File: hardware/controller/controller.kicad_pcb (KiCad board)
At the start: 2 copper layers, 150 x 68 mm, 142 parts, among them J1 Conn_01x05, J2 Conn_01x03, J3 Conn_01x04, J4 USB_B_Micro, J5 Conn_01x03, SW1 ILS_TA180_50, SW10 SW_SPDT, SW2 ILS_TA180_50, SW3 ILS_TA180_50, SW4 ILS_TA180_50, SW5 ILS_TA180_50, SW6 ILS_TA180_50, SW7 ILS_TA180_50, SW8 ILS_TA180_50, SW9 ILS_TA180_50, U1 WS2811, U2 STM32F103C8Tx, U3 WS2811, U4 WS2811, U5 HT75xx-1-SOT89, U6 RFM69CW-915MHZ, U7 TP4056

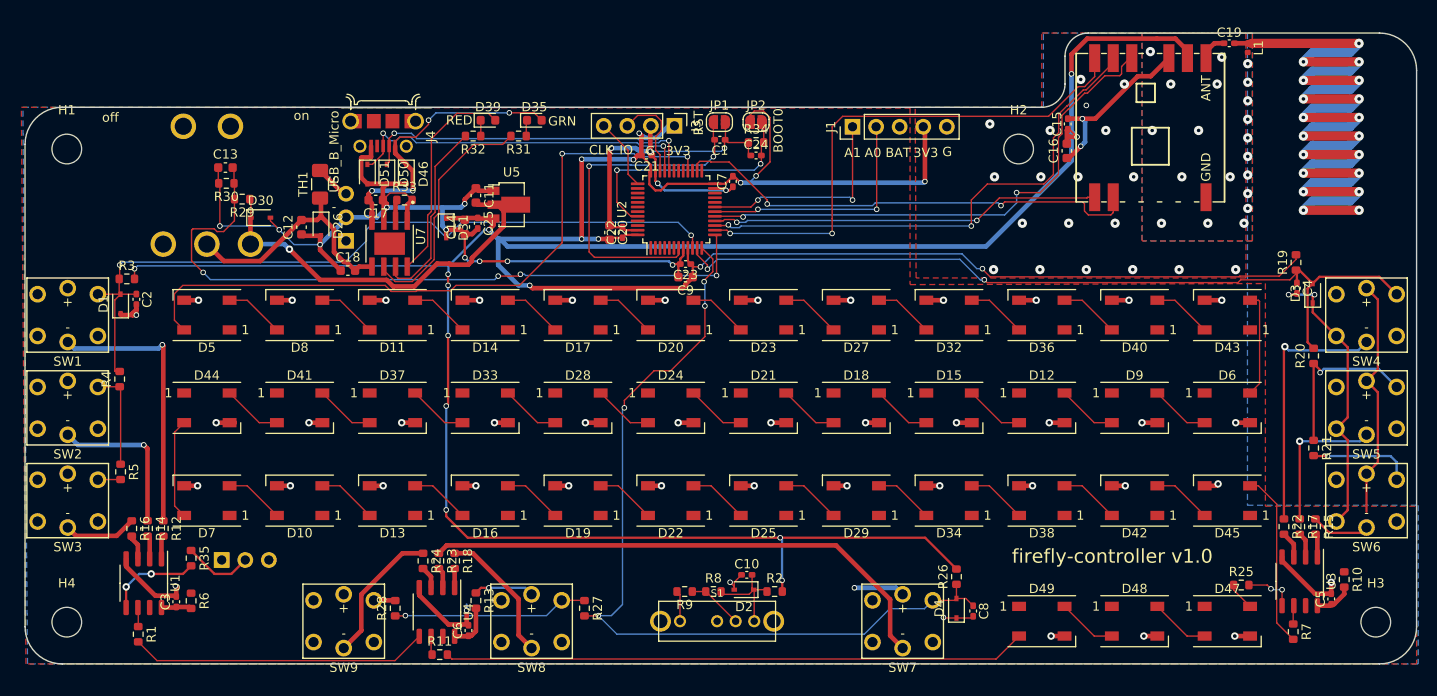
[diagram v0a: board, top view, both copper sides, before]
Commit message: Controller PCB version 1.1
Change-Id: I1cbaa3f158fa0af12788e3f52120070e6be7d808
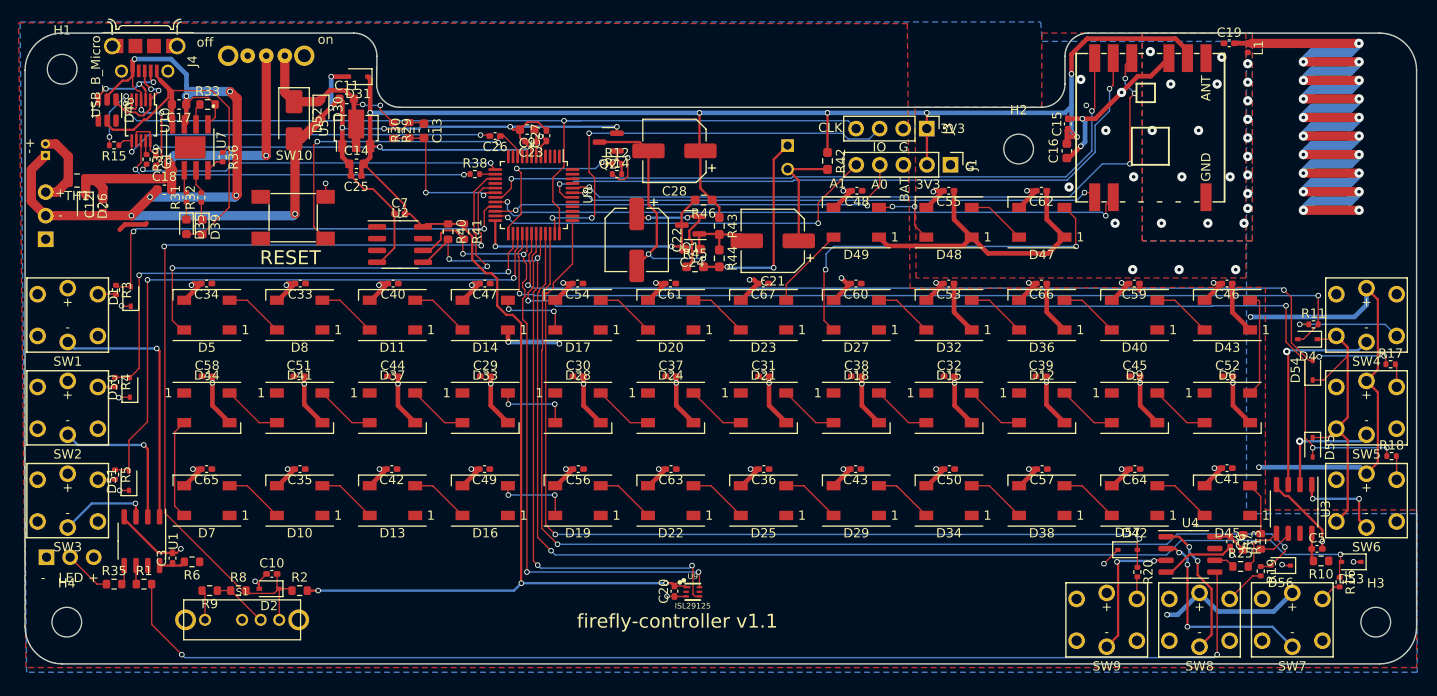
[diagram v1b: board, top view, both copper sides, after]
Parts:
- removed C2, C4, C8: 0.1uF, Capacitor_SMD:C_0402_1005Metric_Pad0.74x0.62mm_HandSolder
- removed D3: D_TVS, Diode_SMD:D_SOD-323
- removed JP1, JP2: SolderJumper_2_Open, Jumper:SolderJumper-2_P1.3mm_Open_RoundedPad1.0x1.5mm
- removed R21, R28: 68k, Resistor_SMD:R_0603_1608Metric
- removed R22, R23, R24: 0R, Resistor_SMD:R_0603_1608Metric
- removed R26: 47k, Resistor_SMD:R_0603_1608Metric
- removed R27, R34: 24k, Resistor_SMD:R_0603_1608Metric
- added C26: 100nF, Capacitor_SMD:C_0402_1005Metric_Pad0.74x0.62mm_HandSolder, F.Cu at (81.1, 100.7)
- added C27: 100nF, Capacitor_SMD:C_0402_1005Metric_Pad0.74x0.62mm_HandSolder, F.Cu at (86.6, 100.7)
- added C28: 100uF, Capacitor_SMD:CP_Elec_6.3x5.4, F.Cu at (100.4, 102.3)
- added C29: 100nF, Capacitor_SMD:C_0402_1005Metric_Pad0.74x0.62mm_HandSolder, F.Cu at (80.0, 126.6)
- added C30: 100nF, Capacitor_SMD:C_0402_1005Metric_Pad0.74x0.62mm_HandSolder, F.Cu at (90.0, 126.6)
- added C31: 100nF, Capacitor_SMD:C_0402_1005Metric_Pad0.74x0.62mm_HandSolder, F.Cu at (110.0, 126.6)
- added C32: 100nF, Capacitor_SMD:C_0402_1005Metric_Pad0.74x0.62mm_HandSolder, F.Cu at (130.0, 126.6)
- added C33: 100nF, Capacitor_SMD:C_0402_1005Metric_Pad0.74x0.62mm_HandSolder, F.Cu at (60.1, 116.6)
- added C34: 100nF, Capacitor_SMD:C_0402_1005Metric_Pad0.74x0.62mm_HandSolder, F.Cu at (50.0, 116.6)
- added C35: 100nF, Capacitor_SMD:C_0402_1005Metric_Pad0.74x0.62mm_HandSolder, F.Cu at (60.0, 136.6)
- added C36: 100nF, Capacitor_SMD:C_0402_1005Metric_Pad0.74x0.62mm_HandSolder, F.Cu at (110.0, 136.6)
- added C37: 100nF, Capacitor_SMD:C_0402_1005Metric_Pad0.74x0.62mm_HandSolder, F.Cu at (100.0, 126.6)
- added C38: 100nF, Capacitor_SMD:C_0402_1005Metric_Pad0.74x0.62mm_HandSolder, F.Cu at (120.0, 126.6)
- added C39: 100nF, Capacitor_SMD:C_0402_1005Metric_Pad0.74x0.62mm_HandSolder, F.Cu at (139.9, 126.6)
- added C40: 100nF, Capacitor_SMD:C_0402_1005Metric_Pad0.74x0.62mm_HandSolder, F.Cu at (70.1, 116.6)
- added C41: 100nF, Capacitor_SMD:C_0402_1005Metric_Pad0.74x0.62mm_HandSolder, F.Cu at (160.0, 136.5)
- added C42: 100nF, Capacitor_SMD:C_0402_1005Metric_Pad0.74x0.62mm_HandSolder, F.Cu at (69.9, 136.6)
- added C43: 100nF, Capacitor_SMD:C_0402_1005Metric_Pad0.74x0.62mm_HandSolder, F.Cu at (119.9, 136.6)
- added C44: 100nF, Capacitor_SMD:C_0402_1005Metric_Pad0.74x0.62mm_HandSolder, F.Cu at (70.0, 126.6)
- added C45: 100nF, Capacitor_SMD:C_0402_1005Metric_Pad0.74x0.62mm_HandSolder, F.Cu at (150.0, 126.6)
- added C46: 100nF, Capacitor_SMD:C_0402_1005Metric_Pad0.74x0.62mm_HandSolder, F.Cu at (160.0, 116.6)
- added C47: 100nF, Capacitor_SMD:C_0402_1005Metric_Pad0.74x0.62mm_HandSolder, F.Cu at (80.0, 116.6)
- added C48: 100nF, Capacitor_SMD:C_0402_1005Metric_Pad0.74x0.62mm_HandSolder, F.Cu at (120.1, 106.6)
- added C49: 100nF, Capacitor_SMD:C_0402_1005Metric_Pad0.74x0.62mm_HandSolder, F.Cu at (79.9, 136.6)
- added C50: 100nF, Capacitor_SMD:C_0402_1005Metric_Pad0.74x0.62mm_HandSolder, F.Cu at (130.0, 136.6)
- added C51: 100nF, Capacitor_SMD:C_0402_1005Metric_Pad0.74x0.62mm_HandSolder, F.Cu at (59.9, 126.6)
- added C52: 100nF, Capacitor_SMD:C_0402_1005Metric_Pad0.74x0.62mm_HandSolder, F.Cu at (160.0, 126.6)
- added C53: 100nF, Capacitor_SMD:C_0402_1005Metric_Pad0.74x0.62mm_HandSolder, F.Cu at (130.0, 116.6)
- added C54: 100nF, Capacitor_SMD:C_0402_1005Metric_Pad0.74x0.62mm_HandSolder, F.Cu at (90.0, 116.6)
- added C55: 100nF, Capacitor_SMD:C_0402_1005Metric_Pad0.74x0.62mm_HandSolder, F.Cu at (130.0, 106.6)
- added C56: 100nF, Capacitor_SMD:C_0402_1005Metric_Pad0.74x0.62mm_HandSolder, F.Cu at (90.0, 136.6)
- added C57: 100nF, Capacitor_SMD:C_0402_1005Metric_Pad0.74x0.62mm_HandSolder, F.Cu at (140.0, 136.6)
- added C58: 100nF, Capacitor_SMD:C_0402_1005Metric_Pad0.74x0.62mm_HandSolder, F.Cu at (50.0, 126.6)
- added C59: 100nF, Capacitor_SMD:C_0402_1005Metric_Pad0.74x0.62mm_HandSolder, F.Cu at (150.0, 116.6)
- added C60: 100nF, Capacitor_SMD:C_0402_1005Metric_Pad0.74x0.62mm_HandSolder, F.Cu at (120.0, 116.6)
- added C61: 100nF, Capacitor_SMD:C_0402_1005Metric_Pad0.74x0.62mm_HandSolder, F.Cu at (100.0, 116.6)
- added C62: 100nF, Capacitor_SMD:C_0402_1005Metric_Pad0.74x0.62mm_HandSolder, F.Cu at (140.0, 106.6)
- added C63: 100nF, Capacitor_SMD:C_0402_1005Metric_Pad0.74x0.62mm_HandSolder, F.Cu at (100.0, 136.6)
- added C64: 100nF, Capacitor_SMD:C_0402_1005Metric_Pad0.74x0.62mm_HandSolder, F.Cu at (150.0, 136.6)
- added C65: 100nF, Capacitor_SMD:C_0402_1005Metric_Pad0.74x0.62mm_HandSolder, F.Cu at (50.0, 136.6)
- added C66: 100nF, Capacitor_SMD:C_0402_1005Metric_Pad0.74x0.62mm_HandSolder, F.Cu at (140.0, 116.6)
- added C67: 100nF, Capacitor_SMD:C_0402_1005Metric_Pad0.74x0.62mm_HandSolder, F.Cu at (110.0, 116.6)
- added D52: D, Diode_SMD:D_SMA, F.Cu at (59.4, 99.0)
- added D53: D_TVS, Diode_SMD:D_SOD-323, F.Cu at (173.3, 146.6)
- added D54: D_TVS, Diode_SMD:D_SOD-323, F.Cu at (169.2, 126.0)
- added D55: D_TVS, Diode_SMD:D_SOD-323, F.Cu at (169.2, 134.2)
- added D56: D_TVS, Diode_SMD:D_SOD-323, F.Cu at (165.8, 147.0)
- added D57: D_TVS, Diode_SMD:D_SOD-323, F.Cu at (149.2, 145.3)
- added J6: Conn_01x02, Homebrew:JST_Micro_1x02_P1.25mm_Horizontal, B.Cu at (32.6, 102.2)
- added MK1: Microphone, Homebrew:MIC_CMA-4544PF-W, B.Cu at (110.6, 103.0)
- added Q1: MMBT2222A 1P, Package_TO_SOT_SMD:SOT-23, F.Cu at (102.1, 110.3)
- added Q2: AO3400A, Package_TO_SOT_SMD:SOT-23, F.Cu at (93.3, 101.3)
- added R36: 1k, Resistor_SMD:R_0402_1005Metric, F.Cu at (51.7, 103.0)
- added R38: 220, Resistor_SMD:R_0402_1005Metric, F.Cu at (78.9, 104.8)
- added R39: 220, Resistor_SMD:R_0402_1005Metric, F.Cu at (43.5, 103.2)
- added R40: 3k3, Resistor_SMD:R_0603_1608Metric, F.Cu at (76.0, 111.0)
- added R41: 3k3, Resistor_SMD:R_0603_1608Metric, F.Cu at (77.7, 111.0)
- added R42: 2k2, Resistor_SMD:R_0603_1608Metric_Pad0.98x0.95mm_HandSolder, F.Cu at (116.9, 103.4)
- added R43: 6k8, Resistor_SMD:R_0603_1608Metric_Pad0.98x0.95mm_HandSolder, F.Cu at (105.2, 110.4)
- added R44: 2k2, Resistor_SMD:R_0603_1608Metric_Pad0.98x0.95mm_HandSolder, F.Cu at (105.2, 113.9)
- added R45: 220, Resistor_SMD:R_0603_1608Metric_Pad0.98x0.95mm_HandSolder, F.Cu at (102.6, 114.8)
- added R46: 1k, Resistor_SMD:R_0603_1608Metric_Pad0.98x0.95mm_HandSolder, F.Cu at (103.5, 107.6)
- added SW11: SW_SPDT, Homebrew:SW_SPDT_SK-12D02-G060, B.Cu at (56.4, 92.0)
- added U10: CH340X, Package_SO:MSOP-10_3x3mm_P0.5mm, F.Cu at (42.9, 99.0)
- added U8: STM32G070CBTx, Package_QFP:LQFP-48_7x7mm_P0.5mm, F.Cu at (85.2, 107.1)
- added U9: ISL29125, Sparkfun_Silicon_Standard:ODFN-6, F.Cu at (102.4, 149.8)
- C1, C10, C15, C23, C25, C3, C5, C6, C7: value 0.1uF -> 100nF
- C11, C12, C13, C14, C16, C17, C18, C9: value 4.7uF -> 10uF
- C20: value 4.7uF -> 100nF; footprint Capacitor_SMD:C_0603_1608Metric -> Capacitor_SMD:C_0402_1005Metric_Pad0.74x0.62mm_HandSolder
- C21, C22: value 0.1uF -> 100uF; footprint Capacitor_SMD:C_0402_1005Metric_Pad0.74x0.62mm_HandSolder -> Capacitor_SMD:CP_Elec_6.3x5.4
- C24: value 0.1uF -> 10nF; footprint Capacitor_SMD:C_0402_1005Metric_Pad0.74x0.62mm_HandSolder -> Capacitor_SMD:C_0603_1608Metric_Pad1.08x0.95mm_HandSolder
- D10, D11, D12, D13, D14, D15, D16, D17, D18, D19, D20, D21, D22, D23, D24, D25, D27, D28, D29, D32, D33, D34, D36, D37, D38, D40, D41, D42, D43, D44, D45, D47, D48, D49, D5, D6, D7, D8, D9: value WS2812B -> WS2812C/W
- D35: value GREEN -> WHITE
- D46: value D_TVS -> SRV05-4-P-T7; footprint Diode_SMD:D_SOD-323 -> Package_TO_SOT_SMD:SOT-23-6
- J5: footprint Connector_PinHeader_2.54mm:PinHeader_1x03_P2.54mm_Horizontal -> Connector_PinHeader_2.54mm:PinHeader_1x03_P2.54mm_Vertical
- R1, R25, R35, R7: value 33R -> 33
- R10, R13, R6: value 100R -> 100
- R11: value 33R -> 1k; footprint Resistor_SMD:R_0603_1608Metric -> Resistor_SMD:R_0402_1005Metric
- R12: value 0R -> 220; footprint Resistor_SMD:R_0603_1608Metric -> Resistor_SMD:R_0402_1005Metric
- R14: value 0R -> 10k; footprint Resistor_SMD:R_0603_1608Metric -> Resistor_SMD:R_0402_1005Metric
- R15: value 0R -> 4k7; footprint Resistor_SMD:R_0603_1608Metric -> Resistor_SMD:R_0402_1005Metric
- R16, R17, R18: value 0R -> 1k; footprint Resistor_SMD:R_0603_1608Metric -> Resistor_SMD:R_0402_1005Metric
- R19, R3: value 47k -> 1k; footprint Resistor_SMD:R_0603_1608Metric -> Resistor_SMD:R_0402_1005Metric
- R20, R4: value 24k -> 1k; footprint Resistor_SMD:R_0603_1608Metric -> Resistor_SMD:R_0402_1005Metric
- R31, R32: footprint Resistor_SMD:R_0603_1608Metric -> Resistor_SMD:R_0402_1005Metric
- R5: value 68k -> 1k; footprint Resistor_SMD:R_0603_1608Metric -> Resistor_SMD:R_0402_1005Metric
- SW1, SW2, SW3, SW4, SW5, SW6, SW7, SW8, SW9: footprint homebrew:SW_CK_TA -> Homebrew:SW_CK_TA
- SW10: value SW_SPDT -> SW_Push; footprint homebrew:ANR11R11P2HQE -> Homebrew:SW_TACTILE_5.1MM_TS-1187A-C-D-B; moved to F.Cu
- TH1: footprint Fuse:Fuse_1206_3216Metric_Pad1.42x1.75mm_HandSolder -> Fuse:Fuse_0805_2012Metric
- U2: value STM32F103C8Tx -> FM24CL16B; footprint Package_QFP:LQFP-48_7x7mm_P0.5mm -> Package_SO:SOIC-8_3.9x4.9mm_P1.27mm
- U7: footprint snapeda:SOP127P600X175-9N -> Homebrew:SOP127P600X175-9N
- moved R15 135.9 mm to (40.0, 101.7), turned to 180 degrees
- moved R16 130.3 mm to (172.1, 148.8)
- moved R18 101.6 mm to (177.7, 135.2), turned to 0 degrees
- moved R11 100.7 mm to (169.3, 121.0)
- moved R13 82.9 mm to (161.7, 144.5)
- moved C6 82.7 mm to (160.3, 144.4), turned to -90 degrees
- moved SW9 82.3 mm to (147.0, 152.8)
- moved U4 81.5 mm to (156.0, 145.8), turned to 0 degrees
- moved SW8 72.0 mm to (157.0, 152.8)
- moved R14 63.4 mm to (94.2, 104.8), turned to 0 degrees
- moved R12 62.7 mm to (94.2, 103.7), turned to 0 degrees
- moved C1 60.8 mm to (44.5, 103.4), turned to -90 degrees
- moved S1 51.2 mm to (53.8, 152.8)
- moved C10 51.2 mm to (57.0, 147.9)
- moved D2 51.2 mm to (56.7, 149.5)
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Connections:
- C1 pad 1: GND -> VCC
- C1 pad 2: Net-(C1-Pad2) -> GND
- C19 pad 1: Net-(C19-Pad1) -> Net-(U6-ANT)
- C21 pad 1: GND -> Net-(MK1-+)
- C21 pad 2: VCC -> Net-(Q1-B)
- C22 pad 1: VCC -> Net-(Q1-E)
- C22 pad 2: GND -> Net-(MK1--)
- C24 pad 1: GND -> Net-(Q1-B)
- C24 pad 2: /BOOT0 -> /MIC_OUT
- D1 pad 2: /SW_LEFT -> /SW_LEFT1
- D23 pad 2: Net-(D23-Pad2) -> Net-(D23-DOUT)
- D27 pad 4: Net-(D23-Pad2) -> Net-(D27-DIN)
- D39 pad 2: Net-(D39-Pad2) -> VBUS
- D4 pad 2: /SW_ACTION -> /SW_RIGHT1
- D46 pad 1: VBUS -> /USB+
- D47 pad 2: Net-(D47-Pad2) -> Net-(D27-DIN)
- D47 pad 4: Net-(D47-Pad4) -> Net-(D47-DIN)
- D48 pad 2: Net-(D48-Pad2) -> Net-(D47-DIN)
- D48 pad 4: Net-(D47-Pad2) -> Net-(D48-DIN)
- D49 pad 2: Net-(D49-Pad2) -> Net-(D48-DIN)
- D49 pad 4: Net-(D48-Pad2) -> Net-(D23-DOUT)
- D50 pad 1: /USB- -> GND
- D50 pad 2: GND -> /SW_LEFT2
- D51 pad 1: /USB+ -> GND
- D51 pad 2: GND -> /SW_LEFT3
- J1 pad 1: /AUX1 -> GND
- J1 pad 2: /AUX0 -> VCC
- J1 pad 4: VCC -> /AUX0
- J1 pad 5: GND -> /AUX1
- J2 pad 1: (no net) -> unconnected-(J2-Pin_1-Pad1)
- J3 pad 4: /SWCLK -> /BOOT0
- J4 pad 4: (no net) -> unconnected-(J4-ID-Pad4)
- J5 pad 1: +BATT -> GND
- J5 pad 3: GND -> +BATT
- R11 pad 2: Net-(D49-Pad2) -> /SW_RIGHT1
- R12 pad 1: /BLED_0 -> /MIC_ENABLE
- R12 pad 2: Net-(R12-Pad2) -> Net-(Q2-G)
- R14 pad 1: /BLED_1 -> GND
- R14 pad 2: Net-(R14-Pad2) -> Net-(Q2-G)
- R15 pad 1: /BLED_5 -> /~{DTR}
- R15 pad 2: Net-(R15-Pad2) -> Net-(U10-~{CTS})
- R16 pad 1: /BLED_2 -> /SW_ACTION1
- R17 pad 1: /BLED_4 -> /SW_RIGHT2
- R18 pad 1: /BLED_7 -> /SW_RIGHT3
- R19 pad 1: /SW_RIGHT -> /SW_ACTION2
- R19 pad 2: VCC -> Net-(R19-Pad2)
- R20 pad 1: Net-(R20-Pad1) -> /SW_ACTION3
- R20 pad 2: /SW_RIGHT -> Net-(R20-Pad2)
- R25 pad 1: Net-(D47-Pad4) -> Net-(U4-DIN)
- R3 pad 1: /SW_LEFT -> /SW_LEFT1
- R3 pad 2: VCC -> Net-(R3-Pad2)
- R4 pad 1: Net-(R4-Pad1) -> /SW_LEFT2
- R4 pad 2: /SW_LEFT -> Net-(R4-Pad2)
- R5 pad 1: Net-(R4-Pad1) -> /SW_LEFT3
- SW1 pad 1: /SW_LEFT -> Net-(R3-Pad2)
- SW1 pad 2: (no net) -> unconnected-(SW1-Pad2)
- SW1 pad 3: (no net) -> unconnected-(SW1-Pad3)
- SW10 pad 1: +BATT -> GND
- SW10 pad 2: /BATT_DIRECT -> Net-(U8-NRST)
- SW2 pad 1: Net-(R4-Pad1) -> Net-(R4-Pad2)
- SW2 pad 2: (no net) -> unconnected-(SW2-Pad2)
- SW2 pad 3: (no net) -> unconnected-(SW2-Pad3)
- SW3 pad 2: (no net) -> unconnected-(SW3-Pad2)
- SW3 pad 3: (no net) -> unconnected-(SW3-Pad3)
- SW4 pad 1: /SW_RIGHT -> unconnected-(SW4-Pad1)
- SW4 pad 2: (no net) -> Net-(R11-Pad1)
- SW4 pad 3: (no net) -> unconnected-(SW4-Pad3)
- SW5 pad 1: Net-(R20-Pad1) -> Net-(R17-Pad2)
- SW5 pad 2: (no net) -> unconnected-(SW5-Pad2)
- SW5 pad 3: (no net) -> unconnected-(SW5-Pad3)
- SW6 pad 1: Net-(R21-Pad2) -> Net-(R18-Pad2)
- SW6 pad 2: (no net) -> unconnected-(SW6-Pad2)
- SW6 pad 3: (no net) -> unconnected-(SW6-Pad3)
- SW7 pad 1: /SW_ACTION -> Net-(R16-Pad2)
- SW7 pad 2: (no net) -> unconnected-(SW7-Pad2)
- SW7 pad 3: (no net) -> unconnected-(SW7-Pad3)
- SW8 pad 1: Net-(R27-Pad1) -> Net-(R19-Pad2)
- SW8 pad 2: (no net) -> unconnected-(SW8-Pad2)
- SW8 pad 3: (no net) -> unconnected-(SW8-Pad3)
- SW9 pad 1: Net-(R28-Pad2) -> Net-(R20-Pad2)
- SW9 pad 2: (no net) -> unconnected-(SW9-Pad2)
- SW9 pad 3: (no net) -> unconnected-(SW9-Pad3)
- U1 pad 1: Net-(R12-Pad2) -> /BLED_0
- U1 pad 2: Net-(R14-Pad2) -> /BLED_1
- U1 pad 3: Net-(R16-Pad2) -> /BLED_2
- U1 pad 7: (no net) -> unconnected-(U1-SET-Pad7)
- U2 pad 1: (no net) -> unconnected-(U2-Pad1)
- U2 pad 2: (no net) -> unconnected-(U2-Pad2)
- U2 pad 3: (no net) -> unconnected-(U2-Pad3)
- U2 pad 4: (no net) -> GND
- U2 pad 5: (no net) -> /SDA
- U2 pad 6: (no net) -> /SCL
- U2 pad 7: Net-(C1-Pad2) -> unconnected-(U2-WP-Pad7)
- U2 pad 8: GND -> VCC
- U3 pad 1: Net-(R15-Pad2) -> /BLED_5
- U3 pad 2: Net-(R17-Pad2) -> /BLED_4
- U3 pad 3: Net-(R22-Pad2) -> /BLED_3
- U3 pad 7: (no net) -> unconnected-(U3-SET-Pad7)
- U4 pad 1: Net-(R18-Pad2) -> /BLED_7
- U4 pad 2: Net-(R23-Pad2) -> /BLED_6
- U4 pad 3: Net-(R24-Pad2) -> /BLED_8
- U4 pad 6: Net-(R11-Pad1) -> Net-(U4-DIN)
- U4 pad 7: (no net) -> unconnected-(U4-SET-Pad7)
- U7 pad 8: Net-(D39-Pad2) -> Net-(U7-CE)
- U7 pad 9: (no net) -> unconnected-(U7-EP-Pad9)
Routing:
- net GND: track 304.3 -> 440.2 mm, vias 102 -> 98
- net VCC: track 423.5 -> 288.8 mm, vias 22 -> 12
- net /SW_ACTION1: track 0.00 -> 124.1 mm, vias 0 -> 2
- net /SW_ACTION2: track 0.00 -> 117.6 mm, vias 0 -> 2
- net /SW_RIGHT3: track 0.00 -> 116.1 mm, vias 0 -> 4
- net /SW_RIGHT2: track 0.00 -> 105.5 mm, vias 0 -> 4
- net /SW_ACTION3: track 0.00 -> 101.9 mm, vias 0 -> 2
- net /SW_RIGHT1: track 0.00 -> 98.8 mm, vias 0 -> 2
- net Net-(U4-DO): track 32.2 -> 129.8 mm, vias 0 -> 2
- net /SW_ACTION: track 93.4 -> 0.00 mm, vias 4 -> 0
- net /SW_RIGHT: track 89.9 -> 0.00 mm, vias 2 -> 0
- net /SW_LEFT: track 83.8 -> 0.00 mm, vias 2 -> 0
- net /SW_MODE: track 10.5 -> 92.8 mm, vias 0 -> 2
- net /SDA: track 0.00 -> 72.3 mm, vias 0 -> 4
- net /SCL: track 0.00 -> 70.8 mm, vias 0 -> 4
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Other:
- outline, holes or cut-outs redrawn
- board text added: "+BAT"
- board text added: "LED"
- board text added: "RESET"
- board text added: "firefly-controller v1.1"
- board text removed: "BOOT0"
- board text removed: "GRN"
- board text removed: "RED"
- board text removed: "RST"
- board text removed: "firefly-controller v1.0"
